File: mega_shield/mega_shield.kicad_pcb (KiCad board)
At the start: 2 copper layers, 301 parts, among them J1 T4140012081-000, J11 T4040014031-000, J13 T4040014031-000, J14 1757242, J15 1757242, J17 T4040014031-000, J19 T4040014031-000, J2 T4140012081-000, J20 T4140012121-000, J3 1757271, J4 T4140012081-000, J5 T4140012081-000, J6 T4140012081-000, J9 T4040014031-000, Q1 2SK3018, Q10 2SK3018, Q11 2SK3018, Q12 2SK3018, Q13 2SK3018, Q14 2SK3018, Q15 2SK3018, Q16 2SK3018, Q17 2SK3018, Q18 2SK3018, Q19 2SK3018, Q2 2SK3018, Q20 2SK3018, Q21 2SK3018, Q22 2SK3018, Q23 2SK3018, Q24 2SK3018, Q25 2SK3018, Q26 2SK3018, Q27 2SK3018, Q28 2SK3018, Q29 2SK3018, Q3 2SK3018, Q30 2SK3018, Q31 2SK3018, Q32 2SK3018, Q33 2SK3018, Q34 2SK3018, Q35 2SK3018, Q36 2SK3018, Q37 2SK3018, Q38 2SK3018, Q39 2SK3018, Q4 2SK3018, Q40 2SK3018, Q41 2SK3018, Q42 2SK3018, Q5 2SK3018, Q6 2SK3018, Q7 2SK3018, Q8 2SK3018, Q9 2SK3018, U1 CS817x22HS, U10 CS817x22HS, U11 CS817x22HS, U12 CS817x22HS, U13 CS817x22HS, U14 CS817x22HS, U15 CS817x22HS, U16 CS817x22HS, U17 CS817x22HS, U18 CS817x22HS, U19 NUP2202, U2 CS817x22HS, U20 NUP2202, U21 NUP2202, U22 NUP2202, U23 NUP2202, U24 CS817x22HS, U25 CS817x22HS, U26 CS817x22HS, U27 CS817x22HS, U28 CS817x22HS, U3 CS817x22HS, U4 CS817x22HS, U5 CS817x22HS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

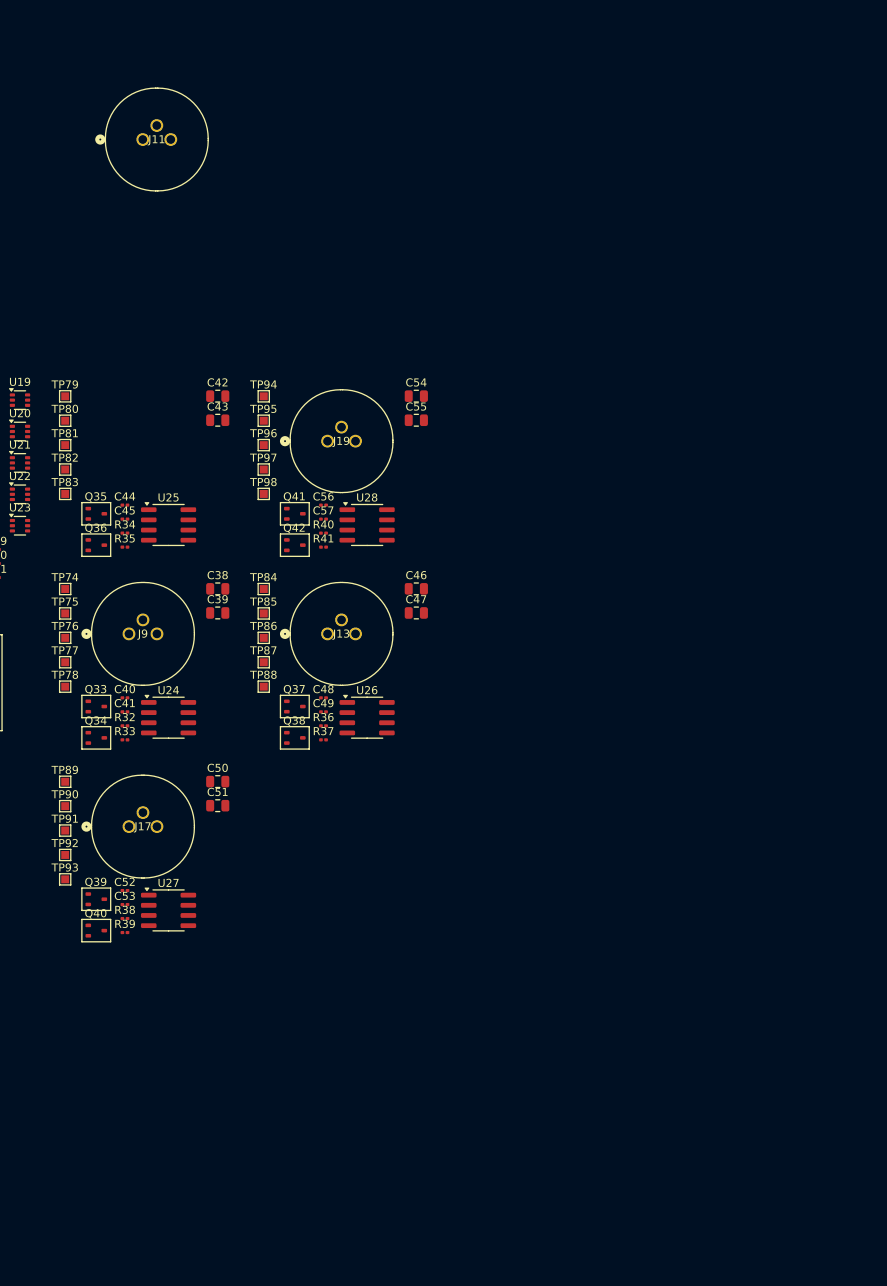
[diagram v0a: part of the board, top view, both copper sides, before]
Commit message: marked the secondary 3pin connectors as included in bom.
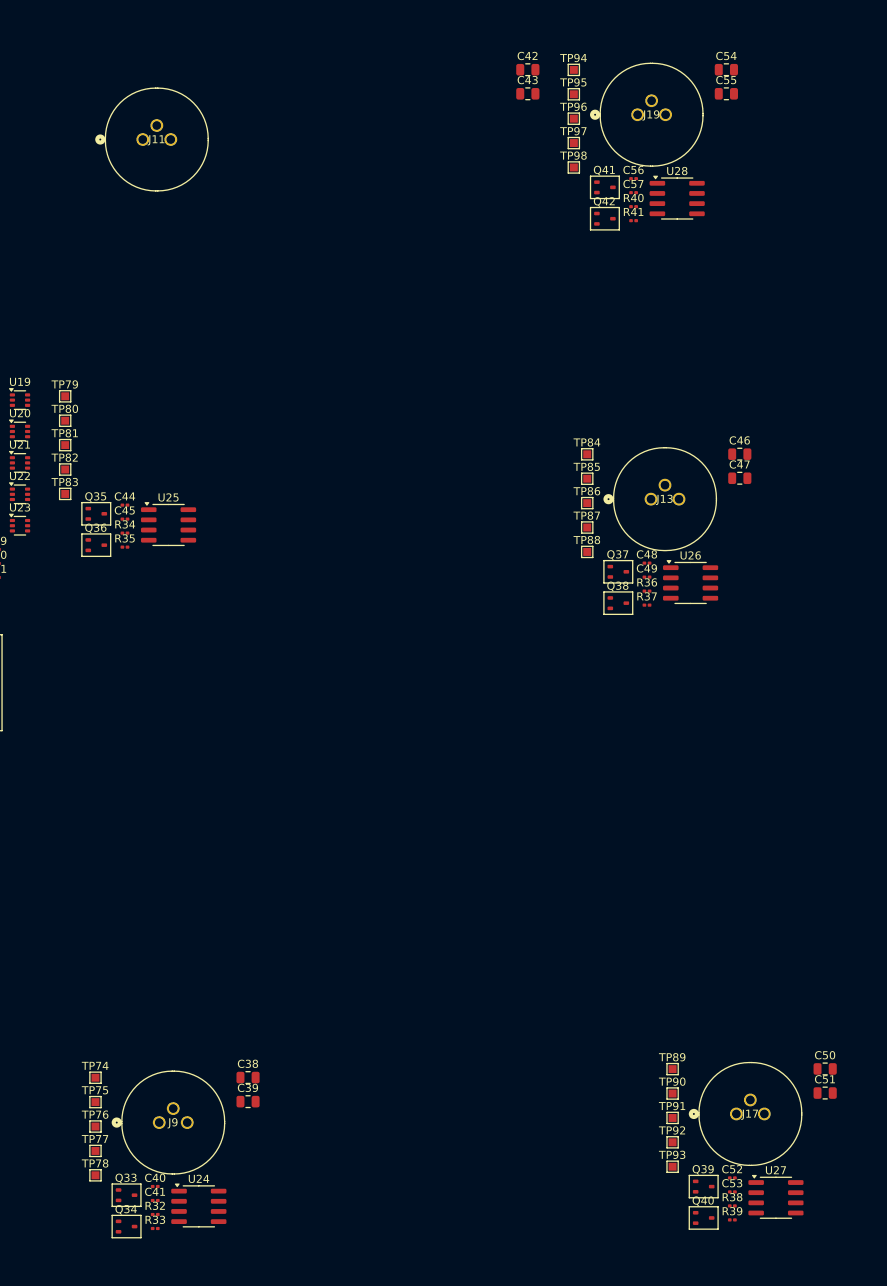
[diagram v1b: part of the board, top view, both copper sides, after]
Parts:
- moved C52 84.0 mm to (-47.8, 190.4)
- moved C53 84.0 mm to (-47.8, 192.2)
- moved R38 84.0 mm to (-47.8, 193.9)
- moved R39 84.0 mm to (-47.8, 195.7)
- moved TP89 84.0 mm to (-55.2, 176.8)
- moved TP91 84.0 mm to (-55.2, 182.9)
- moved J17 84.0 mm to (-47.3, 182.4)
- moved Q39 84.0 mm to (-51.3, 191.5)
- moved TP90 84.0 mm to (-55.2, 179.8)
- moved TP92 84.0 mm to (-55.2, 185.9)
- moved TP93 84.0 mm to (-55.2, 189.0)
- moved U27 84.0 mm to (-42.3, 192.9)
- moved C50 84.0 mm to (-36.2, 176.8)
- moved C51 84.0 mm to (-36.2, 179.8)
- moved Q40 84.0 mm to (-51.3, 195.4)
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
